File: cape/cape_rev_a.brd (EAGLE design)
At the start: 116.4 x 127.2 mm, 35 parts, among them IC1 MAX3042BEUE, IC10 MAX3042BEUE, IC11 MAX3042BEUE, IC12 MAX3042BEUE, IC13 MAX3042BEUE, IC14 MAX3042BEUE, IC15 MAX3042BEUE, IC16 MAX3042BEUE, IC2 MAX3042BEUE, IC3 MAX3042BEUE, IC4 MAX3042BEUE, IC5 MAX3042BEUE, IC6 MAX3042BEUE, IC7 MAX3042BEUE, IC8 MAX3042BEUE, IC9 MAX3042BEUE

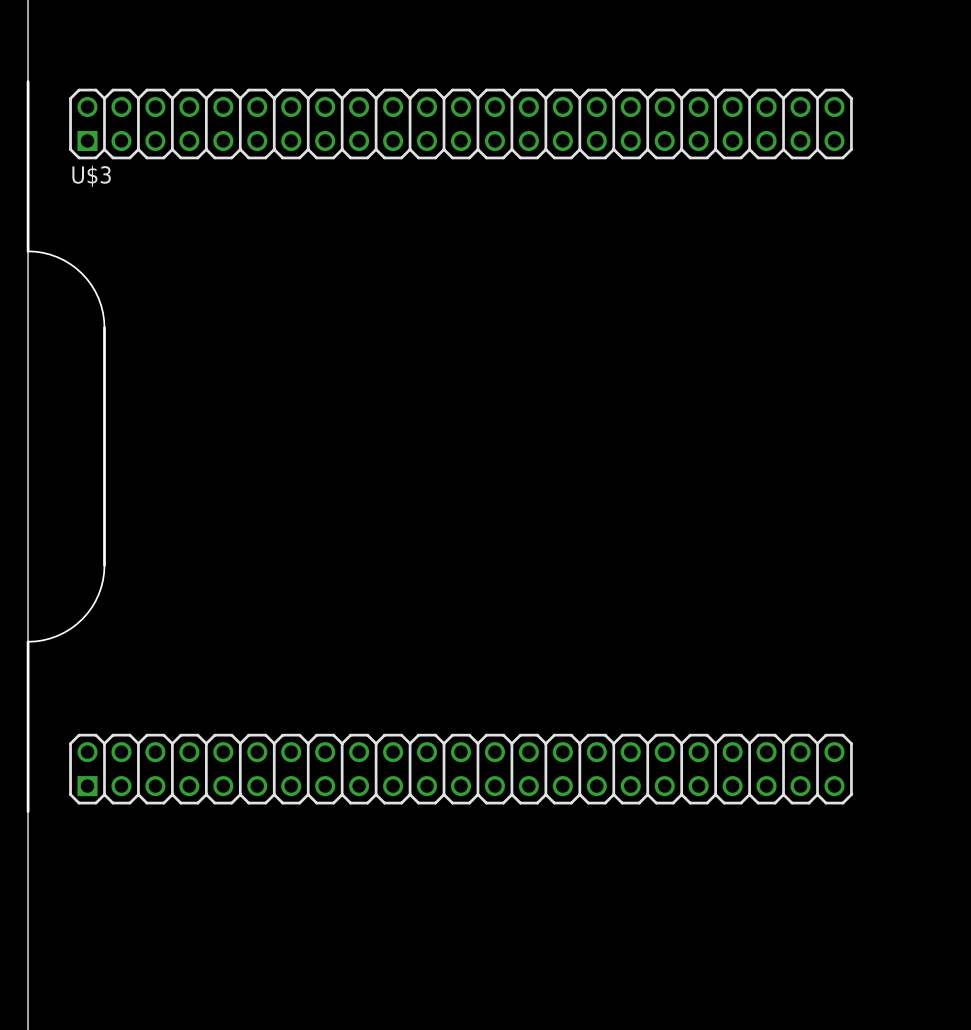
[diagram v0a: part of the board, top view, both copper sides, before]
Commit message: Mostly done with the receiver
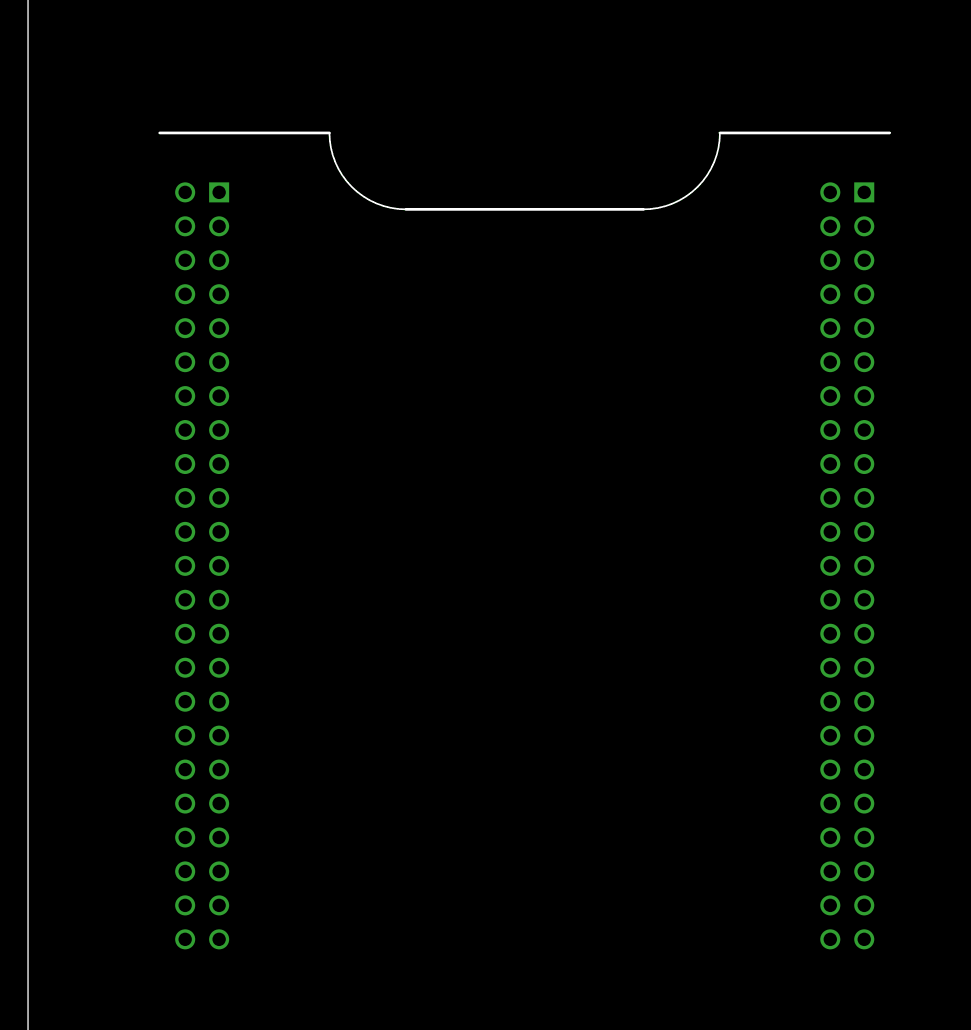
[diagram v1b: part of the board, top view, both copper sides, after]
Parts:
- moved U$3 26.7 mm to (9.83, 105.5), flipped to the bottom, turned to 180 degrees
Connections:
- new net CLOCK0: U$3.27
- new net CLOCK1: U$3.11
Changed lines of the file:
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@@
 <element name="C15" library="SparkFun-Passives" package="0603-CAP" value="0.1uF" x="73.9592" y="106" rot="R180"/>
 <element name="C16" library="SparkFun-Passives" package="0603-CAP" value="0.1uF" x="73.9846" y="112.8862" rot="R180"/>
-<element name="U$3" library="microbuilder" package="BEAGLEBONE_OUTLINE_DOCU" value="BEAGLEBONE_OUTLINEDOCU_OUTLINE" x="-14.619" y="94.765" rot="R270"/>
+<element name="U$3" library="microbuilder" package="BEAGLEBONE_OUTLINE_DOCU" value="BEAGLEBONE_OUTLINEDOCU_OUTLINE" x="9.8322" y="105.5256" rot="MR180"/>
 </elements>
 <signals>
@@
 <wire x1="92.237" y1="5.701" x2="82.0388" y2="13.0908" width="0" layer="19" extent="1-1"/>
 <wire x1="98.587" y1="6.463" x2="92.237" y2="5.701" width="0" layer="19" extent="1-1"/>
-<wire x1="60.311" y1="42.06" x2="73.1854" y2="43.0336" width="0" layer="19" extent="1-1"/>
-<wire x1="60.311" y1="44.6" x2="60.311" y2="42.06" width="0" layer="19" extent="1-1"/>
-<wire x1="57.771" y1="44.6" x2="60.311" y2="44.6" width="0" layer="19" extent="1-1"/>
-<wire x1="57.771" y1="42.06" x2="60.311" y2="42.06" width="0" layer="19" extent="1-1"/>
+<wire x1="62.5372" y1="30.5956" x2="73.1854" y2="43.0336" width="0" layer="19" extent="1-1"/>
+<wire x1="59.9972" y1="30.5956" x2="62.5372" y2="30.5956" width="0" layer="19" extent="1-1"/>
+<wire x1="59.9972" y1="33.1356" x2="59.9972" y2="30.5956" width="0" layer="19" extent="1-1"/>
+<wire x1="62.5372" y1="33.1356" x2="62.5372" y2="30.5956" width="0" layer="19" extent="1-1"/>
 <wire x1="112.303" y1="5.701" x2="98.587" y2="6.463" width="0" layer="19" extent="1-1"/>
-<wire x1="4.431" y1="44.6" x2="57.771" y2="44.6" width="0" layer="19" extent="1-1"/>
-<wire x1="4.431" y1="42.06" x2="4.431" y2="44.6" width="0" layer="19" extent="1-1"/>
-<wire x1="4.431" y1="90.32" x2="4.431" y2="44.6" width="0" layer="19" extent="1-1"/>
-<wire x1="4.431" y1="92.86" x2="4.431" y2="90.32" width="0" layer="19" extent="1-1"/>
+<wire x1="59.9972" y1="86.4756" x2="59.9972" y2="33.1356" width="0" layer="19" extent="1-1"/>
+<wire x1="62.5372" y1="86.4756" x2="59.9972" y2="86.4756" width="0" layer="19" extent="1-1"/>
+<wire x1="14.2772" y1="86.4756" x2="59.9972" y2="86.4756" width="0" layer="19" extent="1-1"/>
+<wire x1="11.7372" y1="86.4756" x2="14.2772" y2="86.4756" width="0" layer="19" extent="1-1"/>
 </signal>
 <signal name="VCC">
@@
 <contactref element="U$3" pad="49"/>
 <contactref element="U$3" pad="50"/>
-<wire x1="6.971" y1="42.06" x2="6.971" y2="44.6" width="0" layer="19" extent="1-1"/>
+<wire x1="62.5372" y1="83.9356" x2="59.9972" y2="83.9356" width="0" layer="19" extent="1-1"/>
 </signal>
 <signal name="VDD_5V">
 <contactref element="U$3" pad="51"/>
 <contactref element="U$3" pad="52"/>
-<wire x1="9.511" y1="42.06" x2="9.511" y2="44.6" width="0" layer="19" extent="1-1"/>
+<wire x1="62.5372" y1="81.3956" x2="59.9972" y2="81.3956" width="0" layer="19" extent="1-1"/>
 </signal>
 <signal name="SYS_5V">
 <contactref element="U$3" pad="53"/>
 <contactref element="U$3" pad="54"/>
-<wire x1="12.051" y1="42.06" x2="12.051" y2="44.6" width="0" layer="19" extent="1-1"/>
+<wire x1="62.5372" y1="78.8556" x2="59.9972" y2="78.8556" width="0" layer="19" extent="1-1"/>
 </signal>
 <signal name="VDD_ADC">
@@
 <wire x1="76.2032" y1="9.1908" x2="76.2032" y2="16.0702" width="0" layer="19" extent="1-1"/>
 </signal>
+<signal name="CLOCK1">
+<contactref element="U$3" pad="11"/>
+</signal>
+<signal name="CLOCK0">
+<contactref element="U$3" pad="27"/>
+</signal>
 </signals>
